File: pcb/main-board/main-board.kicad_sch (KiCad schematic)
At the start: 23 parts, among them J1 Conn_01x07, J2 Conn_01x05, P1 USB_C_Plug_USB2.0, SW1 PROG, SW1 RESET, SW1 SW_Push, U1 ESP32-WROOM-32, U2 PC817, U3 PC817, U4 PC817, U5 PC817, U6 AMS1117

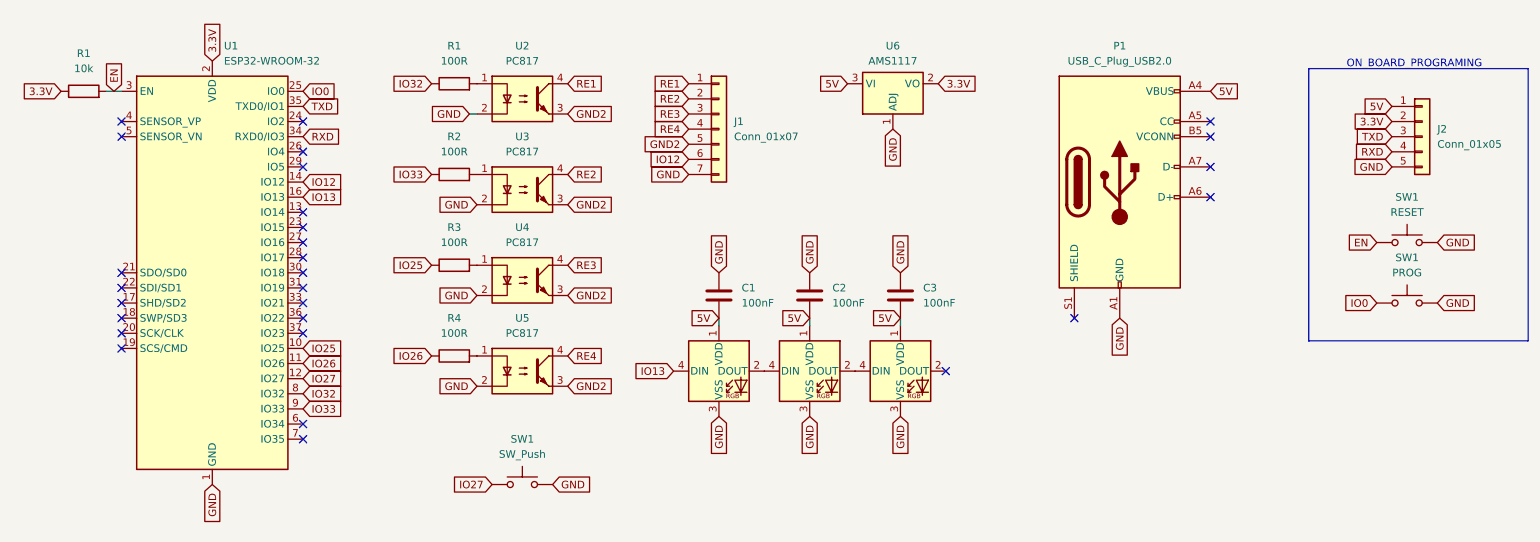
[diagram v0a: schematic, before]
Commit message: New PCB & case
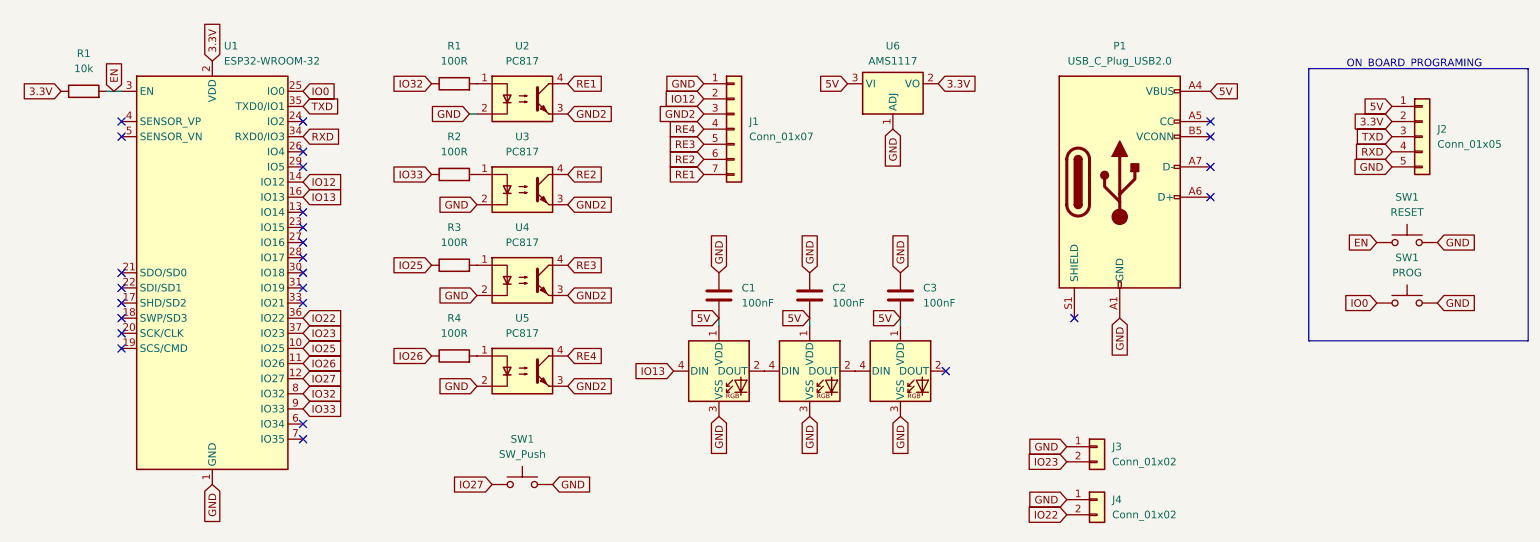
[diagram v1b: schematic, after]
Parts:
- added J3, J4: Conn_01x02, Connector_JST:JST_XH_S2B-XH-A_1x02_P2.50mm_Horizontal, symbol Connector_Generic:Conn_01x02
- J1: footprint Connector_PinSocket_2.54mm:PinSocket_1x07_P2.54mm_Horizontal -> Connector_PinHeader_2.54mm:PinHeader_1x07_P2.54mm_Horizontal
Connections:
- net GND: now also J1.1 (Pin_1), J3.1 (Pin_1), J4.1 (Pin_1); no longer J1.7 (Pin_7)
- net GND2: now also J1.3 (Pin_3); no longer J1.5 (Pin_5)
- net IO12: now also J1.2 (Pin_2); no longer J1.6 (Pin_6)
- net RE1: now also J1.7 (Pin_7); no longer J1.1 (Pin_1)
- net RE2: now also J1.6 (Pin_6); no longer J1.2 (Pin_2)
- net RE3: now also J1.5 (Pin_5); no longer J1.3 (Pin_3)
- net IO22: now reaches U1.36 (IO22)
- net IO22: now also J4.2 (Pin_2)
- net IO23: now reaches U1.37 (IO23)
- net IO23: now also J3.2 (Pin_2)
- no-connect marks 28 -> 26
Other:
- moved on the sheet: J1
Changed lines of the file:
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@@
   (no_connect (at 59.69 87.63))
   (no_connect (at 212.09 44.45))
-  (no_connect (at 59.69 72.39))
   (no_connect (at 29.21 67.31))
   (no_connect (at 212.09 39.37))
@@
   (no_connect (at 212.09 36.83))
   (no_connect (at 59.69 44.45))
-  (no_connect (at 59.69 69.85))
   (no_connect (at 59.69 52.07))
   (no_connect (at 59.69 36.83))
@@
     )
   )
-  (global_label "GND" (shape input) (at 124.46 45.72 180) (fields_autoplaced)
-    (effects (font (size 1.27 1.27)) (justify right))
-    (property "Intersheetrefs" "${INTERSHEET_REFS}" (at 117.6837 45.72 0)
+  (global_label "GND" (shape input) (at 127 30.48 180) (fields_autoplaced)
+    (effects (font (size 1.27 1.27)) (justify right))
+    (property "Intersheetrefs" "${INTERSHEET_REFS}" (at 120.2237 30.48 0)
       (effects (font (size 1.27 1.27)) (justify right) hide)
     )
@@
     )
   )
-  (global_label "GND2" (shape input) (at 124.46 40.64 180) (fields_autoplaced)
-    (effects (font (size 1.27 1.27)) (justify right))
-    (property "Intersheetrefs" "${INTERSHEET_REFS}" (at 116.4742 40.64 0)
+  (global_label "GND2" (shape input) (at 127 35.56 180) (fields_autoplaced)
+    (effects (font (size 1.27 1.27)) (justify right))
+    (property "Intersheetrefs" "${INTERSHEET_REFS}" (at 119.0142 35.56 0)
       (effects (font (size 1.27 1.27)) (justify right) hide)
     )
@@
     )
   )
-  (global_label "RE3" (shape input) (at 124.46 35.56 180) (fields_autoplaced)
-    (effects (font (size 1.27 1.27)) (justify right))
-    (property "Intersheetrefs" "${INTERSHEET_REFS}" (at 117.9257 35.56 0)
+  (global_label "RE3" (shape input) (at 127 40.64 180) (fields_autoplaced)
+    (effects (font (size 1.27 1.27)) (justify right))
+    (property "Intersheetrefs" "${INTERSHEET_REFS}" (at 120.4657 40.64 0)
       (effects (font (size 1.27 1.27)) (justify right) hide)
     )
@@
     )
   )
+  (global_label "GND" (shape input) (at 187.96 91.44 180) (fields_autoplaced)
+    (effects (font (size 1.27 1.27)) (justify right))
+    (property "Intersheetrefs" "${INTERSHEET_REFS}" (at 181.1837 91.44 0)
+      (effects (font (size 1.27 1.27)) (justify right) hide)
+    )
+  )
   (global_label "IO13" (shape input) (at 121.92 78.74 180) (fields_autoplaced)
     (effects (font (size 1.27 1.27)) (justify right))
@@
     )
   )
+  (global_label "IO22" (shape input) (at 187.96 102.87 180) (fields_autoplaced)
+    (effects (font (size 1.27 1.27)) (justify right))
+    (property "Intersheetrefs" "${INTERSHEET_REFS}" (at 180.6999 102.87 0)
+      (effects (font (size 1.27 1.27)) (justify right) hide)
+    )
+  )
   (global_label "RE4" (shape input) (at 104.14 76.2 0) (fields_autoplaced)
     (effects (font (size 1.27 1.27)) (justify left))
@@
     )
   )
-  (global_label "RE4" (shape input) (at 124.46 38.1 180) (fields_autoplaced)
-    (effects (font (size 1.27 1.27)) (justify right))
-    (property "Intersheetrefs" "${INTERSHEET_REFS}" (at 117.9257 38.1 0)
+  (global_label "RE4" (shape input) (at 127 38.1 180) (fields_autoplaced)
+    (effects (font (size 1.27 1.27)) (justify right))
+    (property "Intersheetrefs" "${INTERSHEET_REFS}" (at 120.4657 38.1 0)
       (effects (font (size 1.27 1.27)) (justify right) hide)
     )
@@
     )
   )
+  (global_label "IO23" (shape input) (at 59.69 72.39 0) (fields_autoplaced)
+    (effects (font (size 1.27 1.27)) (justify left))
+    (property "Intersheetrefs" "${INTERSHEET_REFS}" (at 66.9501 72.39 0)
+      (effects (font (size 1.27 1.27)) (justify left) hide)
+    )
+  )
   (global_label "5V" (shape input) (at 242.57 34.29 180) (fields_autoplaced)
     (effects (font (size 1.27 1.27)) (justify right))
@@
     )
   )
-  (global_label "RE1" (shape input) (at 124.46 30.48 180) (fields_autoplaced)
-    (effects (font (size 1.27 1.27)) (justify right))
-    (property "Intersheetrefs" "${INTERSHEET_REFS}" (at 117.9257 30.48 0)
+  (global_label "RE1" (shape input) (at 127 45.72 180) (fields_autoplaced)
+    (effects (font (size 1.27 1.27)) (justify right))
+    (property "Intersheetrefs" "${INTERSHEET_REFS}" (at 120.4657 45.72 0)
       (effects (font (size 1.27 1.27)) (justify right) hide)
     )
@@
     )
   )
-  (global_label "RE2" (shape input) (at 124.46 33.02 180) (fields_autoplaced)
-    (effects (font (size 1.27 1.27)) (justify right))
-    (property "Intersheetrefs" "${INTERSHEET_REFS}" (at 117.9257 33.02 0)
+  (global_label "RE2" (shape input) (at 127 43.18 180) (fields_autoplaced)
+    (effects (font (size 1.27 1.27)) (justify right))
+    (property "Intersheetrefs" "${INTERSHEET_REFS}" (at 120.4657 43.18 0)
       (effects (font (size 1.27 1.27)) (justify right) hide)
     )
@@
     )
   )
+  (global_label "IO22" (shape input) (at 59.69 69.85 0) (fields_autoplaced)
+    (effects (font (size 1.27 1.27)) (justify left))
+    (property "Intersheetrefs" "${INTERSHEET_REFS}" (at 66.9501 69.85 0)
+      (effects (font (size 1.27 1.27)) (justify left) hide)
+    )
+  )
+  (global_label "GND" (shape input) (at 187.96 100.33 180) (fields_autoplaced)
+    (effects (font (size 1.27 1.27)) (justify right))
+    (property "Intersheetrefs" "${INTERSHEET_REFS}" (at 181.1837 100.33 0)
+      (effects (font (size 1.27 1.27)) (justify right) hide)
+    )
+  )
   (global_label "IO32" (shape input) (at 81.28 30.48 180) (fields_autoplaced)
     (effects (font (size 1.27 1.27)) (justify right))
@@
     )
   )
+  (global_label "IO23" (shape input) (at 187.96 93.98 180) (fields_autoplaced)
+    (effects (font (size 1.27 1.27)) (justify right))
+    (property "Intersheetrefs" "${INTERSHEET_REFS}" (at 180.6999 93.98 0)
+      (effects (font (size 1.27 1.27)) (justify right) hide)
+    )
+  )
   (global_label "5V" (shape input) (at 151.13 30.48 180) (fields_autoplaced)
     (effects (font (size 1.27 1.27)) (justify right))
@@
     )
   )
-  (global_label "IO12" (shape input) (at 124.46 43.18 180) (fields_autoplaced)
-    (effects (font (size 1.27 1.27)) (justify right))
-    (property "Intersheetrefs" "${INTERSHEET_REFS}" (at 117.1999 43.18 0)
+  (global_label "IO12" (shape input) (at 127 33.02 180) (fields_autoplaced)
+    (effects (font (size 1.27 1.27)) (justify right))
+    (property "Intersheetrefs" "${INTERSHEET_REFS}" (at 119.7399 33.02 0)
       (effects (font (size 1.27 1.27)) (justify right) hide)
     )
@@
     )
   )
-  (symbol (lib_id "Connector_Generic:Conn_01x07") (at 129.54 38.1 0) (unit 1)
-    (in_bom yes) (on_board yes) (dnp no) (fields_autoplaced)
-    (property "Reference" "J1" (at 132.08 36.83 0)
-      (effects (font (size 1.27 1.27)) (justify left))
-    )
-    (property "Value" "Conn_01x07" (at 132.08 39.37 0)
-      (effects (font (size 1.27 1.27)) (justify left))
-    )
-    (property "Footprint" "Connector_PinSocket_2.54mm:PinSocket_1x07_P2.54mm_Horizontal" (at 129.54 38.1 0)
-      (effects (font (size 1.27 1.27)) hide)
-    )
-    (property "Datasheet" "~" (at 129.54 38.1 0)
+  (symbol (lib_id "Connector_Generic:Conn_01x07") (at 132.08 38.1 0) (unit 1)
+    (in_bom yes) (on_board yes) (dnp no) (fields_autoplaced)
+    (property "Reference" "J1" (at 134.62 36.83 0)
+      (effects (font (size 1.27 1.27)) (justify left))
+    )
+    (property "Value" "Conn_01x07" (at 134.62 39.37 0)
+      (effects (font (size 1.27 1.27)) (justify left))
+    )
+    (property "Footprint" "Connector_PinHeader_2.54mm:PinHeader_1x07_P2.54mm_Horizontal" (at 132.08 38.1 0)
+      (effects (font (size 1.27 1.27)) hide)
+    )
+    (property "Datasheet" "~" (at 132.08 38.1 0)
       (effects (font (size 1.27 1.27)) hide)
     )
@@
         (path "/e93d6aa3-928d-4df9-b25b-21169669388b"
           (reference "U2") (unit 1)
+        )
+      )
+    )
+  )
+  (symbol (lib_id "Connector_Generic:Conn_01x02") (at 193.04 100.33 0) (unit 1)
+    (in_bom yes) (on_board yes) (dnp no) (fields_autoplaced)
+    (property "Reference" "J4" (at 195.58 100.33 0)
+      (effects (font (size 1.27 1.27)) (justify left))
+    )
+    (property "Value" "Conn_01x02" (at 195.58 102.87 0)
+      (effects (font (size 1.27 1.27)) (justify left))
+    )
+    (property "Footprint" "Connector_JST:JST_XH_S2B-XH-A_1x02_P2.50mm_Horizontal" (at 193.04 100.33 0)
+      (effects (font (size 1.27 1.27)) hide)
+    )
+    (property "Datasheet" "~" (at 193.04 100.33 0)
+      (effects (font (size 1.27 1.27)) hide)
+    )
+    (pin "1")
+    (pin "2")
+    (instances
+      (project "main-board"
+        (path "/e93d6aa3-928d-4df9-b25b-21169669388b"
+          (reference "J4") (unit 1)
         )
       )
@@
         )
       )
+    )
+  )
+  (symbol (lib_id "Connector_Generic:Conn_01x02") (at 193.04 91.44 0) (unit 1)
+    (in_bom yes) (on_board yes) (dnp no) (fields_autoplaced)
+    (property "Reference" "J3" (at 195.58 91.44 0)
+      (effects (font (size 1.27 1.27)) (justify left))
+    )
+    (property "Value" "Conn_01x02" (at 195.58 93.98 0)
+      (effects (font (size 1.27 1.27)) (justify left))
+    )
+    (property "Footprint" "Connector_JST:JST_XH_S2B-XH-A_1x02_P2.50mm_Horizontal" (at 193.04 91.44 0)
+      (effects (font (size 1.27 1.27)) hide)
+    )
+    (property "Datasheet" "~" (at 193.04 91.44 0)
+      (effects (font (size 1.27 1.27)) hide)
+    )
+    (pin "1")
+    (pin "2")
+    (instances
+      (project "main-board"
+        (path "/e93d6aa3-928d-4df9-b25b-21169669388b"
+          (reference "J3") (unit 1)
+        )
+      )
